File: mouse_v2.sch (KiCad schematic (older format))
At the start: 110 parts, among them J1 HC05 Header, J2 Serial Debug Header, J3 HC05_Key Jump, J4 Conn_ARM_JTAG_SWD_10, J5 SWD Header, J6 Conn_01x02_Female, J7 Conn_01x02_Female, J8 Conn_01x02_Female, J9 Conn_01x02_Female, M1 M1_Conn, M2 M2_Conn, M3 M1_Conn_Alt, M4 M2_Conn_Alt, Q0 Q_Photo_NPN, Q1 Q_Photo_NPN, Q10 Q_NMOS_GSD, Q11 Q_NMOS_GSD, Q12 Q_NMOS_GSD, Q2 Q_Photo_NPN, Q3 Q_Photo_NPN, Q4 Q_NMOS_SGD, Q5 Q_NMOS_SGD, Q6 Q_NMOS_SGD, Q7 Q_NMOS_SGD, Q8 Q_NMOS_SGD, Q9 Q_NMOS_GSD, SW1 SW, U1 YAAJ_BluePill_SWD_Breakout, U2 L293D, U3 LM1085-5.0, U4 APE8865Y5-33-HF-3

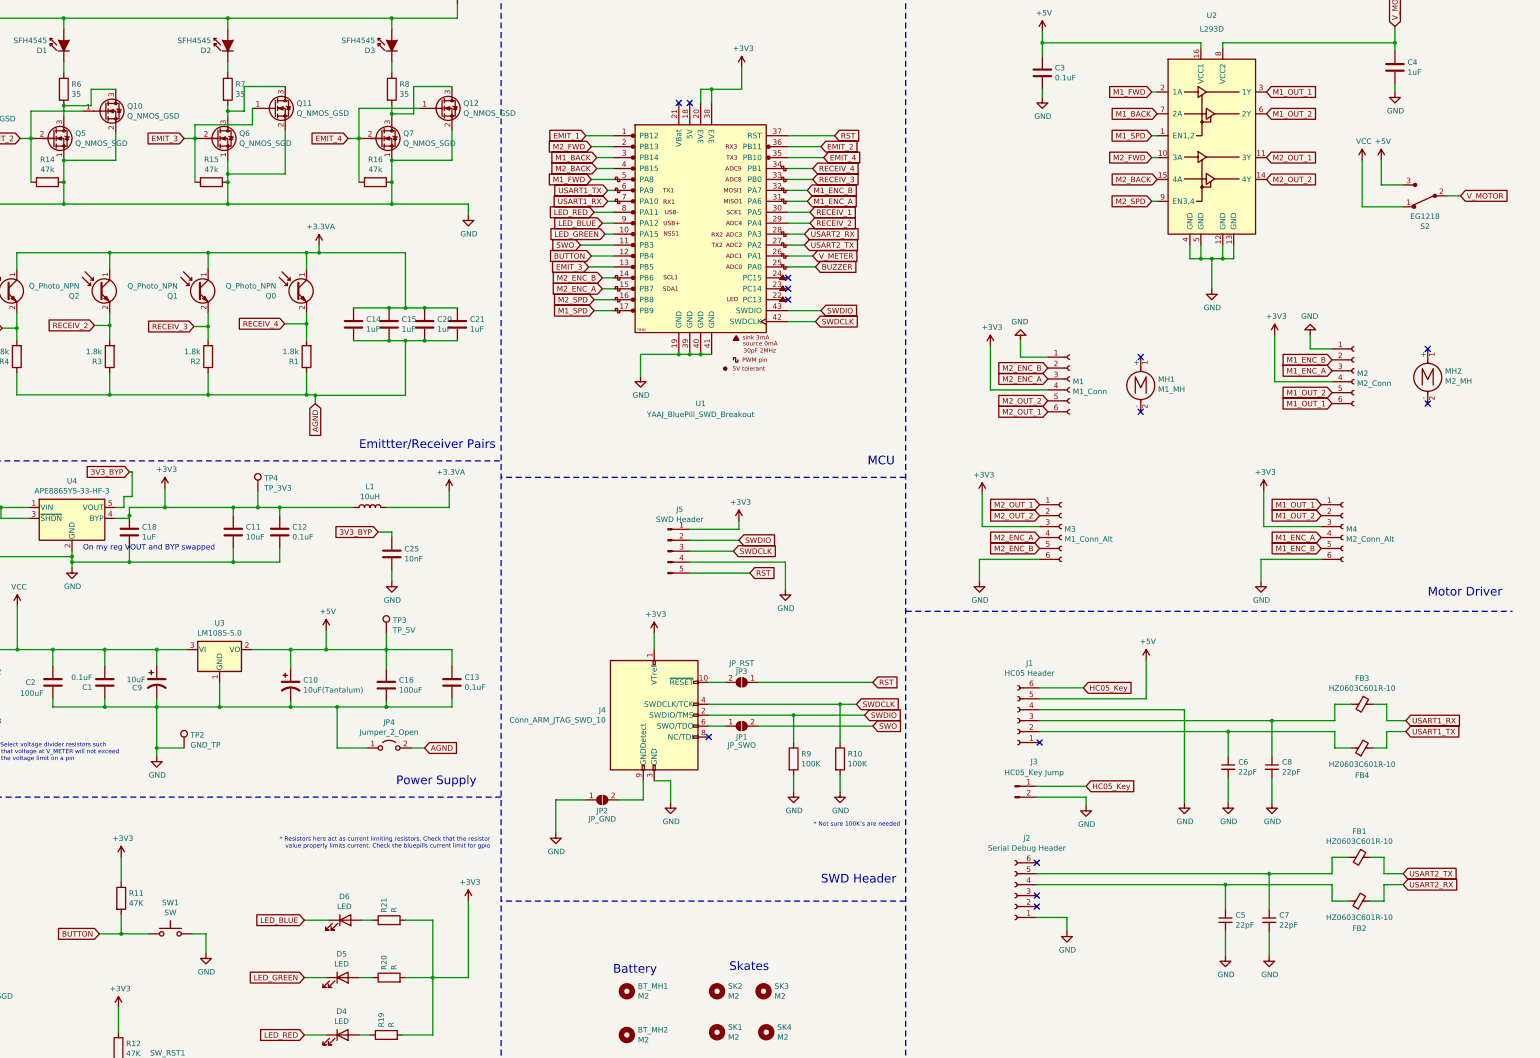
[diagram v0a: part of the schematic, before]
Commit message: changes for v0.1 wip
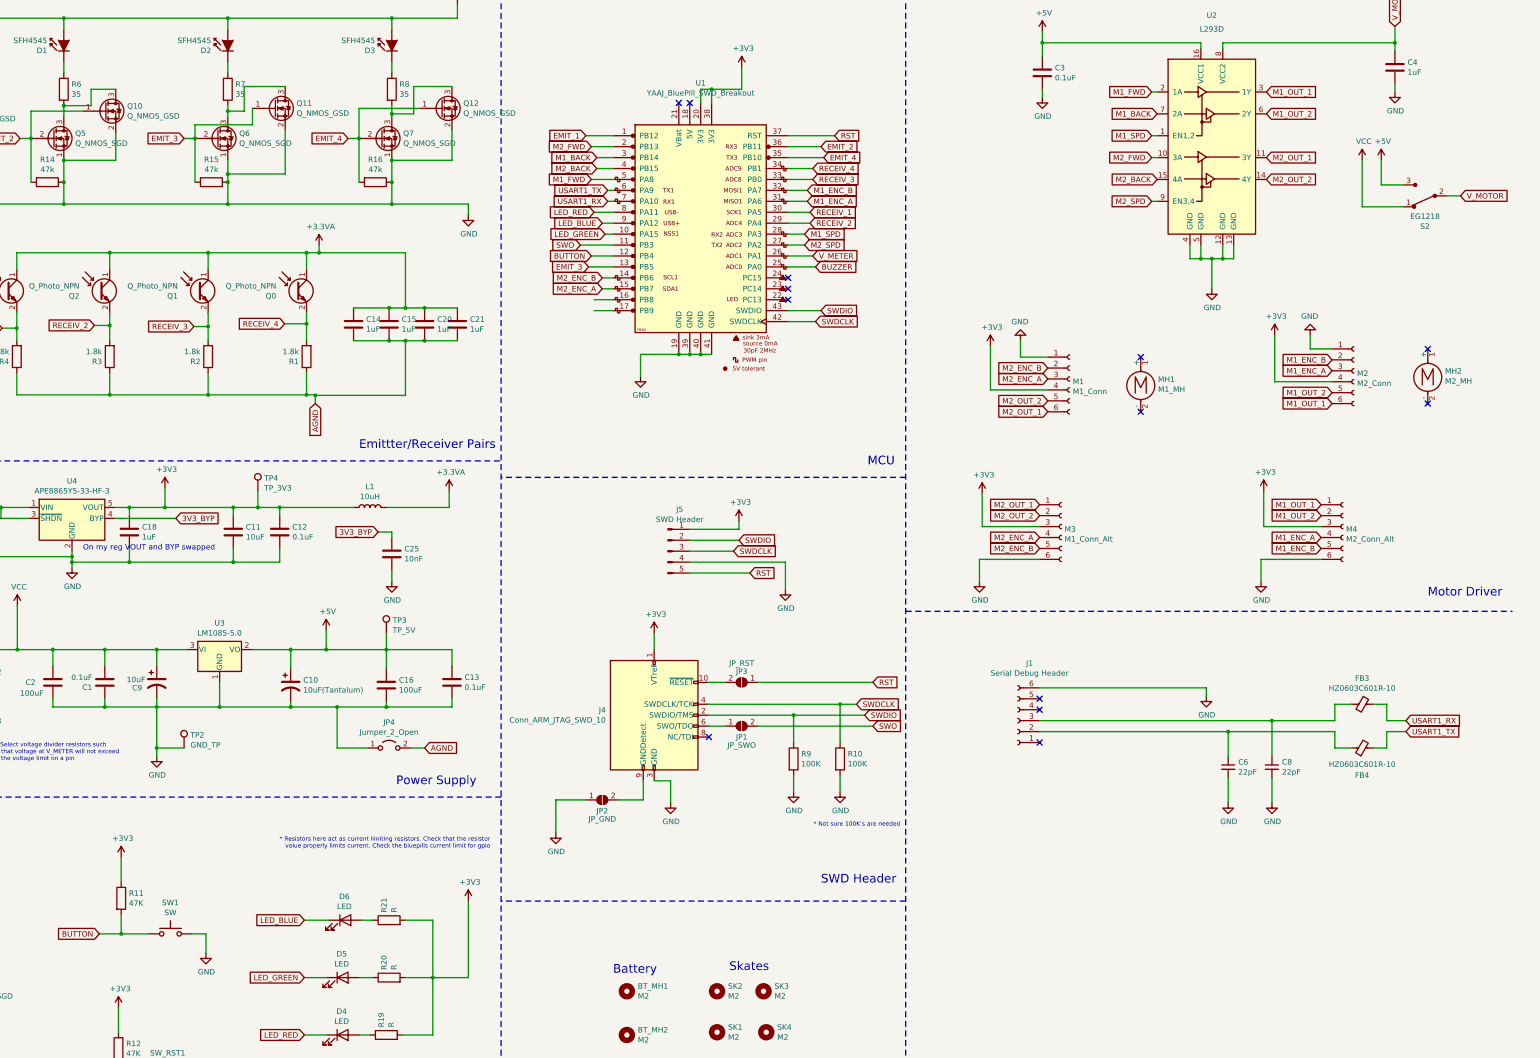
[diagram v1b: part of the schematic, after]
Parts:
- removed C5, C7: 22pF, Capacitor_SMD:C_0603_1608Metric_Pad1.08x0.95mm_HandSolder, symbol Device:C_Small
- removed FB1, FB2: HZ0603C601R-10, Resistor_SMD:R_0603_1608Metric_Pad0.98x0.95mm_HandSolder, symbol Device:FerriteBead_Small
- removed J2: Serial Debug Header, Connector_PinHeader_2.54mm:PinHeader_1x06_P2.54mm_Vertical, symbol Connector:Conn_01x06_Female
- removed J3: HC05_Key Jump, Connector_PinHeader_2.54mm:PinHeader_1x02_P2.54mm_Vertical, symbol Connector:Conn_01x02_Male
- J1: value HC05 Header -> Serial Debug Header
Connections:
- net HC05_Key is gone; now on net GND: J1.6 (Pin_6)
- net USART2_RX is gone; now on net M1_SPD: U1.28 (PA3)
- net USART2_TX is gone; now on net M2_SPD: U1.27 (PA2)
- net +3V3: now also U4.5 (VOUT); no longer U4.4 (BYP)
- net +5V: no longer J1.5 (Pin_5)
- net 3V3_BYP: now also U4.4 (BYP); no longer U4.5 (VOUT)
- net GND: no longer J1.4 (Pin_4)
- net M1_SPD: no longer U1.17 (PB9)
- net M2_SPD: no longer U1.16 (PB8)
- no-connect marks 14 -> 13
